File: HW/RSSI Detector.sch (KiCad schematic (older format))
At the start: 28 parts, among them P1 SMA, P2 SMA, U1 AD8319, U2 AD8319, U3 Teensy3.2, X1 CX3099NL

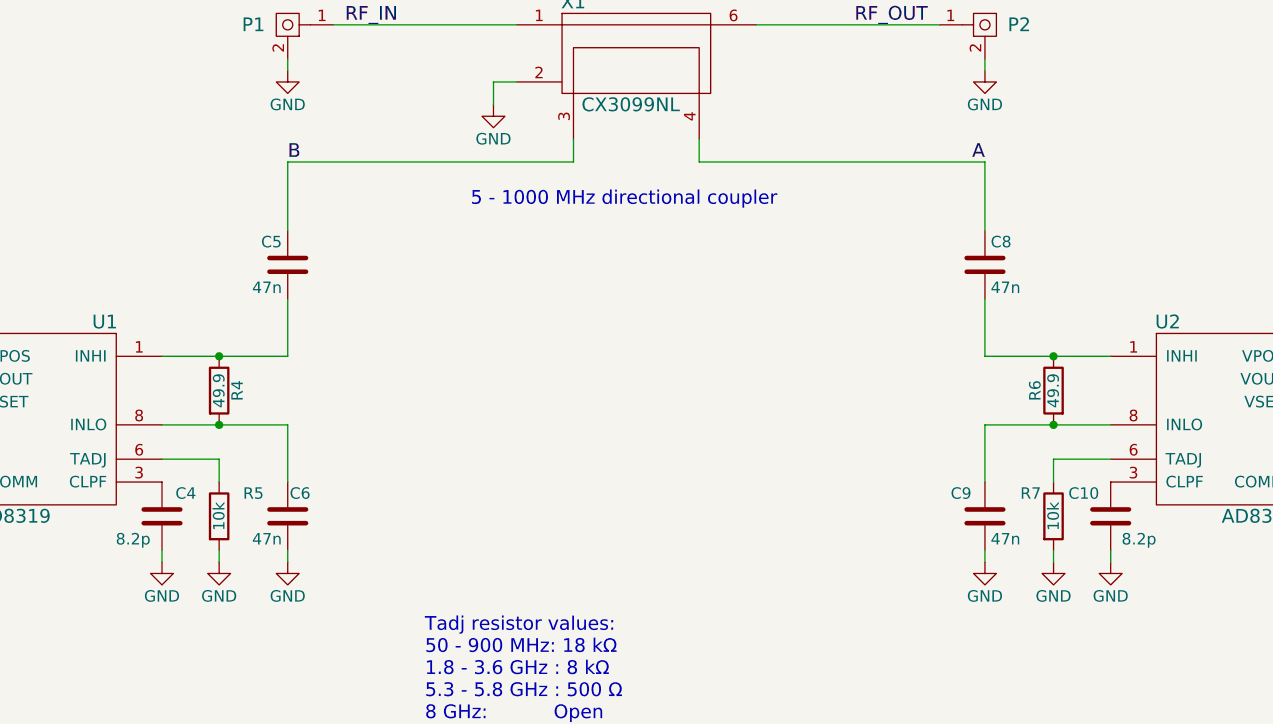
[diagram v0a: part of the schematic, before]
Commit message: prelim placement
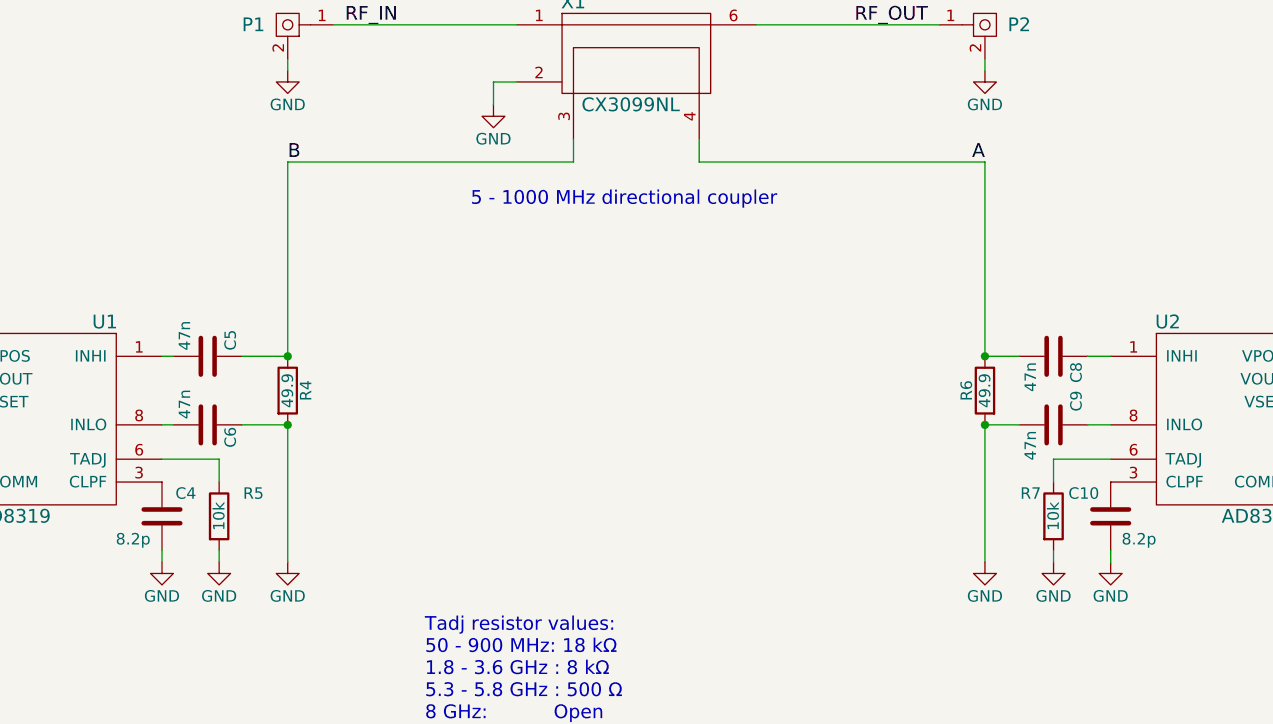
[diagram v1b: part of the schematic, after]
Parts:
- C10, C12, C3, C4: footprint vna:C_0402b -> vna:C_0603b
- C5, C6, C8, C9: footprint VNA:C_0402b -> vna:C_0402b
- R1, R10: footprint VNA:R_0402b -> Resistors_SMD:R_0603
- R2, R3, R5, R7, R8, R9: footprint vna:R_0603b -> Resistors_SMD:R_0603
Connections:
- net A: now also C8.2, R6.1; no longer C8.1
- net B: now also R4.1
- net GND: now also C6.1, R4.2, R6.2; no longer C6.2
- net at C5.2, U1.1 (INHI): no longer R4.1
- net at C9.1, U2.8 (INLO): no longer R6.2
- new net: C8.1, U2.1 (INHI)
- new net: C6.2, U1.8 (INLO)
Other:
- moved on the sheet: C5, C6, C8, C9, R4, R6
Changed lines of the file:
@@
 L R R4
 U 1 1 59C23EFC
-P 3900 5050
-F 0 "R4" V 3980 5050 50  0000 C CNN
-F 1 "49.9" V 3900 5050 50  0000 C CNN
-F 2 "vna:R_0402b" V 3830 5050 30  0001 C CNN
-F 3 "" H 3900 5050 30  0000 C CNN
-	1    3900 5050
+P 4200 5050
+F 0 "R4" V 4280 5050 50  0000 C CNN
+F 1 "49.9" V 4200 5050 50  0000 C CNN
+F 2 "vna:R_0402b" V 4130 5050 30  0001 C CNN
+F 3 "" H 4200 5050 30  0000 C CNN
+	1    4200 5050
 	1    0    0    -1
 $EndComp
@@
 A
 $Comp
-L C C8
-U 1 1 59C23F21
-P 7250 4500
-F 0 "C8" H 7275 4600 50  0000 L CNN
-F 1 "47n" H 7275 4400 50  0000 L CNN
-F 2 "VNA:C_0402b" H 7288 4350 30  0001 C CNN
-F 3 "" H 7250 4500 60  0000 C CNN
-	1    7250 4500
-	1    0    0    -1
-$EndComp
-$Comp
-L C C5
-U 1 1 59C23F6A
-P 4200 4500
-F 0 "C5" H 4225 4600 50  0000 L CNN
-F 1 "47n" H 4225 4400 50  0000 L CNN
-F 2 "VNA:C_0402b" H 4238 4350 30  0001 C CNN
-F 3 "" H 4200 4500 60  0000 C CNN
-	1    4200 4500
-	-1   0    0    -1
-$EndComp
-$Comp
 L R R1
 U 1 1 59C23F92
@@
 F 0 "R1" V 2030 5000 50  0000 C CNN
 F 1 "1k" V 1950 5000 50  0000 C CNN
-F 2 "VNA:R_0402b" V 1880 5000 30  0001 C CNN
+F 2 "Resistors_SMD:R_0603" V 1880 5000 30  0001 C CNN
 F 3 "" H 1950 5000 30  0000 C CNN
 	1    1950 5000
@@
 L R R6
 U 1 1 59C2507D
-P 7550 5050
-F 0 "R6" V 7630 5050 50  0000 C CNN
-F 1 "49.9" V 7550 5050 50  0000 C CNN
-F 2 "vna:R_0402b" V 7480 5050 30  0001 C CNN
-F 3 "" H 7550 5050 30  0000 C CNN
-	1    7550 5050
+P 7250 5050
+F 0 "R6" V 7330 5050 50  0000 C CNN
+F 1 "49.9" V 7250 5050 50  0000 C CNN
+F 2 "vna:R_0402b" V 7180 5050 30  0001 C CNN
+F 3 "" H 7250 5050 30  0000 C CNN
+	1    7250 5050
 	-1   0    0    -1
 $EndComp
@@
 F 0 "R10" V 9580 5000 50  0000 C CNN
 F 1 "1k" V 9500 5000 50  0000 C CNN
-F 2 "VNA:R_0402b" V 9430 5000 30  0001 C CNN
+F 2 "Resistors_SMD:R_0603" V 9430 5000 30  0001 C CNN
 F 3 "" H 9500 5000 30  0000 C CNN
 	1    9500 5000
@@
 F 0 "C3" V 2150 4450 50  0000 L CNN
 F 1 "100p" V 2250 4650 50  0000 L CNN
-F 2 "vna:C_0402b" H 2238 4450 50  0001 C CNN
+F 2 "vna:C_0603b" H 2238 4450 50  0001 C CNN
 F 3 "" H 2200 4600 50  0001 C CNN
 	1    2200 4600
@@
 	6000 3950 6000 4050
 Wire Wire Line
-	7250 4650 7250 4900
-Wire Wire Line
-	7250 4900 7800 4900
+	7250 4050 7250 4900
 Wire Wire Line
 	6000 4050 7250 4050
 Wire Wire Line
-	7250 4050 7250 4350
-Wire Wire Line
-	4200 4900 4200 4650
-Wire Wire Line
-	3650 4900 4200 4900
+	4200 4050 4200 4900
 Wire Wire Line
 	2100 5000 2650 5000
@@
 Wire Wire Line
 	5450 4050 4200 4050
-Wire Wire Line
-	4200 4050 4200 4350
 Wire Wire Line
 	1700 5000 1700 5100
@@
 Wire Wire Line
 	4200 3600 4200 3650
-Connection ~ 3900 4900
-Wire Wire Line
-	3650 5200 4200 5200
-Connection ~ 7550 4900
-Wire Wire Line
-	7250 5200 7800 5200
+Connection ~ 4200 4900
+Connection ~ 7250 4900
+Wire Wire Line
+	7250 5200 7400 5200
 Wire Wire Line
 	2650 5100 2600 5100
@@
 F 0 "C12" H 9275 4650 50  0000 L CNN
 F 1 "100p" H 9275 4450 50  0000 L CNN
-F 2 "vna:C_0402b" H 9288 4400 50  0001 C CNN
+F 2 "vna:C_0603b" H 9288 4400 50  0001 C CNN
 F 3 "" H 9250 4550 50  0001 C CNN
 	1    9250 4550
@@
 L C C6
 U 1 1 59C28F3F
-P 4200 5600
-F 0 "C6" H 4100 5700 50  0000 L CNN
-F 1 "47n" H 4225 5500 50  0000 L CNN
-F 2 "VNA:C_0402b" H 4238 5450 30  0001 C CNN
-F 3 "" H 4200 5600 60  0000 C CNN
-	1    4200 5600
-	-1   0    0    -1
-$EndComp
-Wire Wire Line
-	4200 5200 4200 5450
-Connection ~ 3900 5200
+P 3850 5200
+F 0 "C6" H 3750 5300 50  0000 L CNN
+F 1 "47n" H 3875 5100 50  0000 L CNN
+F 2 "vna:C_0402b" H 3888 5050 30  0001 C CNN
+F 3 "" H 3850 5200 60  0000 C CNN
+	1    3850 5200
+	0    1    -1   0
+$EndComp
+Wire Wire Line
+	4200 5200 4200 5800
+Connection ~ 4200 5200
 $Comp
 L C C9
 U 1 1 59C29280
-P 7250 5600
-F 0 "C9" H 7100 5700 50  0000 L CNN
-F 1 "47n" H 7275 5500 50  0000 L CNN
-F 2 "VNA:C_0402b" H 7288 5450 30  0001 C CNN
-F 3 "" H 7250 5600 60  0000 C CNN
-	1    7250 5600
-	1    0    0    -1
-$EndComp
-Wire Wire Line
-	7250 5200 7250 5450
-Connection ~ 7550 5200
+P 7550 5200
+F 0 "C9" H 7400 5300 50  0000 L CNN
+F 1 "47n" H 7575 5100 50  0000 L CNN
+F 2 "vna:C_0402b" H 7588 5050 30  0001 C CNN
+F 3 "" H 7550 5200 60  0000 C CNN
+	1    7550 5200
+	0    1    1    0
+$EndComp
+Wire Wire Line
+	7250 5200 7250 5800
+Connection ~ 7250 5200
 $Comp
 L R R5
@@
 F 0 "R5" H 4050 5700 50  0000 C CNN
 F 1 "10k" V 3900 5600 50  0000 C CNN
-F 2 "vna:R_0603b" V 3830 5600 30  0001 C CNN
+F 2 "Resistors_SMD:R_0603" V 3830 5600 30  0001 C CNN
 F 3 "" H 3900 5600 30  0000 C CNN
 	1    3900 5600
@@
 F 0 "R7" H 7450 5700 50  0000 C CNN
 F 1 "10k" V 7550 5600 50  0000 C CNN
-F 2 "vna:R_0603b" V 7480 5600 30  0001 C CNN
+F 2 "Resistors_SMD:R_0603" V 7480 5600 30  0001 C CNN
 F 3 "" H 7550 5600 30  0000 C CNN
 	1    7550 5600
@@
 F 0 "R2" V 2330 5450 50  0000 C CNN
 F 1 "10k" V 2250 5450 50  0000 C CNN
-F 2 "vna:R_0603b" V 2180 5450 30  0001 C CNN
+F 2 "Resistors_SMD:R_0603" V 2180 5450 30  0001 C CNN
 F 3 "" H 2250 5450 30  0000 C CNN
 	1    2250 5450
@@
 F 0 "R3" V 2530 5100 50  0000 C CNN
 F 1 "10k" V 2450 5100 50  0000 C CNN
-F 2 "vna:R_0603b" V 2380 5100 30  0001 C CNN
+F 2 "Resistors_SMD:R_0603" V 2380 5100 30  0001 C CNN
 F 3 "" H 2450 5100 30  0000 C CNN
 	1    2450 5100
@@
 F 0 "R9" V 9280 5450 50  0000 C CNN
 F 1 "10k" V 9200 5450 50  0000 C CNN
-F 2 "vna:R_0603b" V 9130 5450 30  0001 C CNN
+F 2 "Resistors_SMD:R_0603" V 9130 5450 30  0001 C CNN
 F 3 "" H 9200 5450 30  0000 C CNN
 	1    9200 5450
@@
 F 0 "R8" V 9080 5100 50  0000 C CNN
 F 1 "10k" V 9000 5100 50  0000 C CNN
-F 2 "vna:R_0603b" V 8930 5100 30  0001 C CNN
+F 2 "Resistors_SMD:R_0603" V 8930 5100 30  0001 C CNN
 F 3 "" H 9000 5100 30  0000 C CNN
 	1    9000 5100
@@
 F 0 "C4" H 3500 5500 50  0000 L CNN
 F 1 "8.2p" H 3700 5700 50  0000 L CNN
-F 2 "vna:C_0402b" H 3688 5450 50  0001 C CNN
+F 2 "vna:C_0603b" H 3688 5450 50  0001 C CNN
 F 3 "" H 3650 5600 50  0001 C CNN
 	1    3650 5600
@@
 F 0 "C10" H 7850 5500 50  0000 L CNN
 F 1 "8.2p" H 7600 5700 50  0000 L CNN
-F 2 "vna:C_0402b" H 7838 5450 50  0001 C CNN
+F 2 "vna:C_0603b" H 7838 5450 50  0001 C CNN
 F 3 "" H 7800 5600 50  0001 C CNN
 	1    7800 5600
@@
 Wire Wire Line
 	3900 5750 3900 5800
-Wire Wire Line
-	4200 5750 4200 5800
 $Comp
 L GND #PWR014
@@
 Wire Wire Line
 	7550 5750 7550 5800
-Wire Wire Line
-	7250 5750 7250 5800
 Wire Wire Line
 	8800 5450 8850 5450
@@
 NoConn ~ 8600 3300
 NoConn ~ 8600 3400
+$Comp
+L C C5
+U 1 1 59C23F6A
+P 3850 4900
+F 0 "C5" H 3875 5000 50  0000 L CNN
+F 1 "47n" H 3875 4800 50  0000 L CNN
+F 2 "vna:C_0402b" H 3888 4750 30  0001 C CNN
+F 3 "" H 3850 4900 60  0000 C CNN
+	1    3850 4900
+	0    1    -1   0
+$EndComp
+Wire Wire Line
+	4200 4900 4000 4900
+Wire Wire Line
+	3700 4900 3650 4900
+Wire Wire Line
+	3650 5200 3700 5200
+Wire Wire Line
+	4000 5200 4200 5200
+$Comp
+L C C8
+U 1 1 59C23F21
+P 7550 4900
+F 0 "C8" H 7575 5000 50  0000 L CNN
+F 1 "47n" H 7575 4800 50  0000 L CNN
+F 2 "vna:C_0402b" H 7588 4750 30  0001 C CNN
+F 3 "" H 7550 4900 60  0000 C CNN
+	1    7550 4900
+	0    1    1    0
+$EndComp
+Wire Wire Line
+	7250 4900 7400 4900
+Wire Wire Line
+	7700 4900 7800 4900
+Wire Wire Line
+	7700 5200 7800 5200
 $EndSCHEMATC
